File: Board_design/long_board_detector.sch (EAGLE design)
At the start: 57 parts, among them IC1 TL072P, IC2 78L05Z, IC3 LM393N, Q1 BC549, Q2 BC549, Q3 BC549, Q4 BC549, X1 22-23-2021, X2 22-23-2021

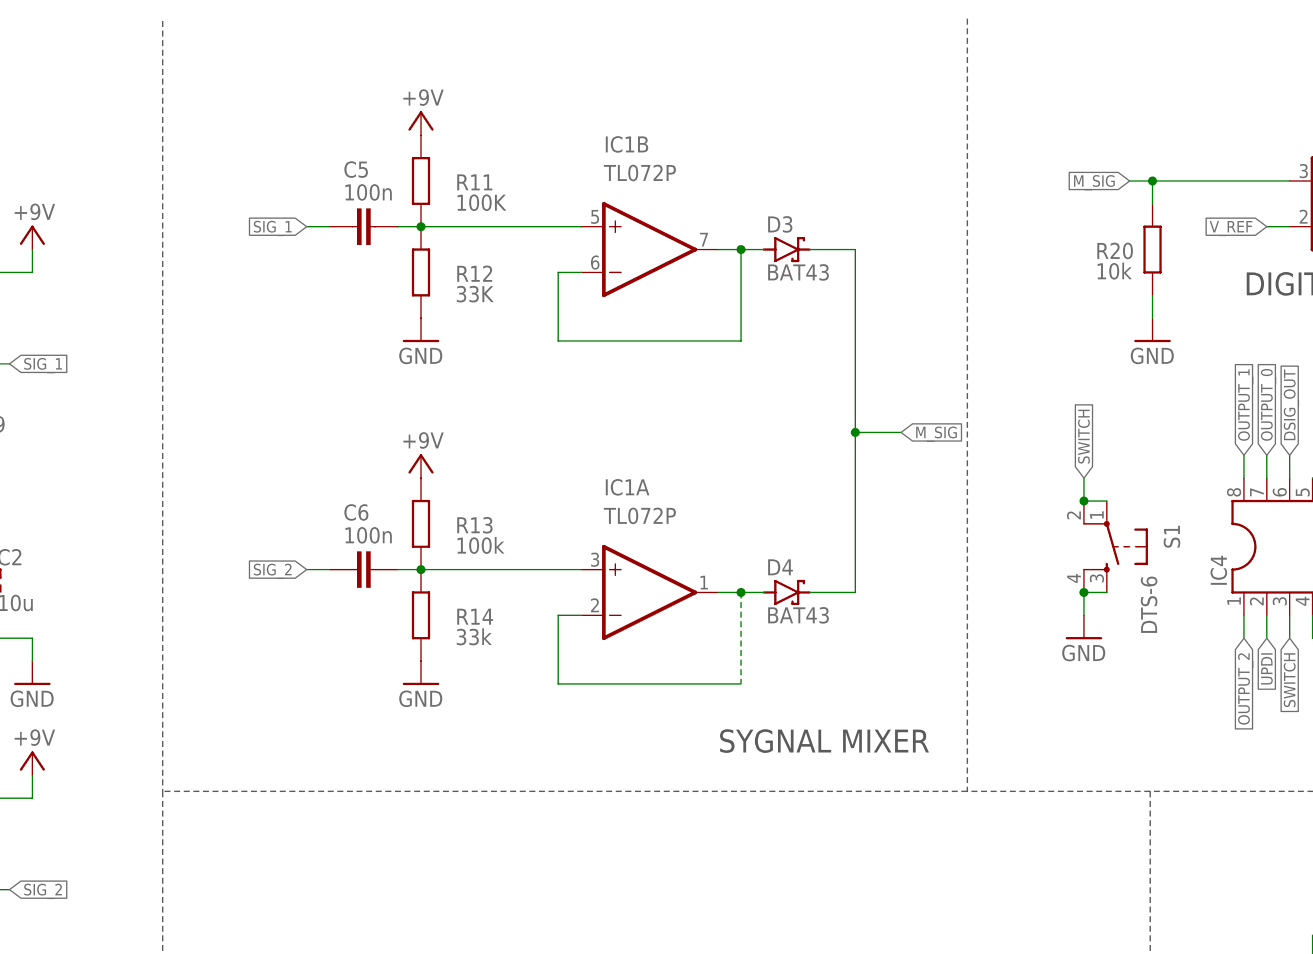
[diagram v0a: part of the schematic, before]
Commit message: Readme and brd design update
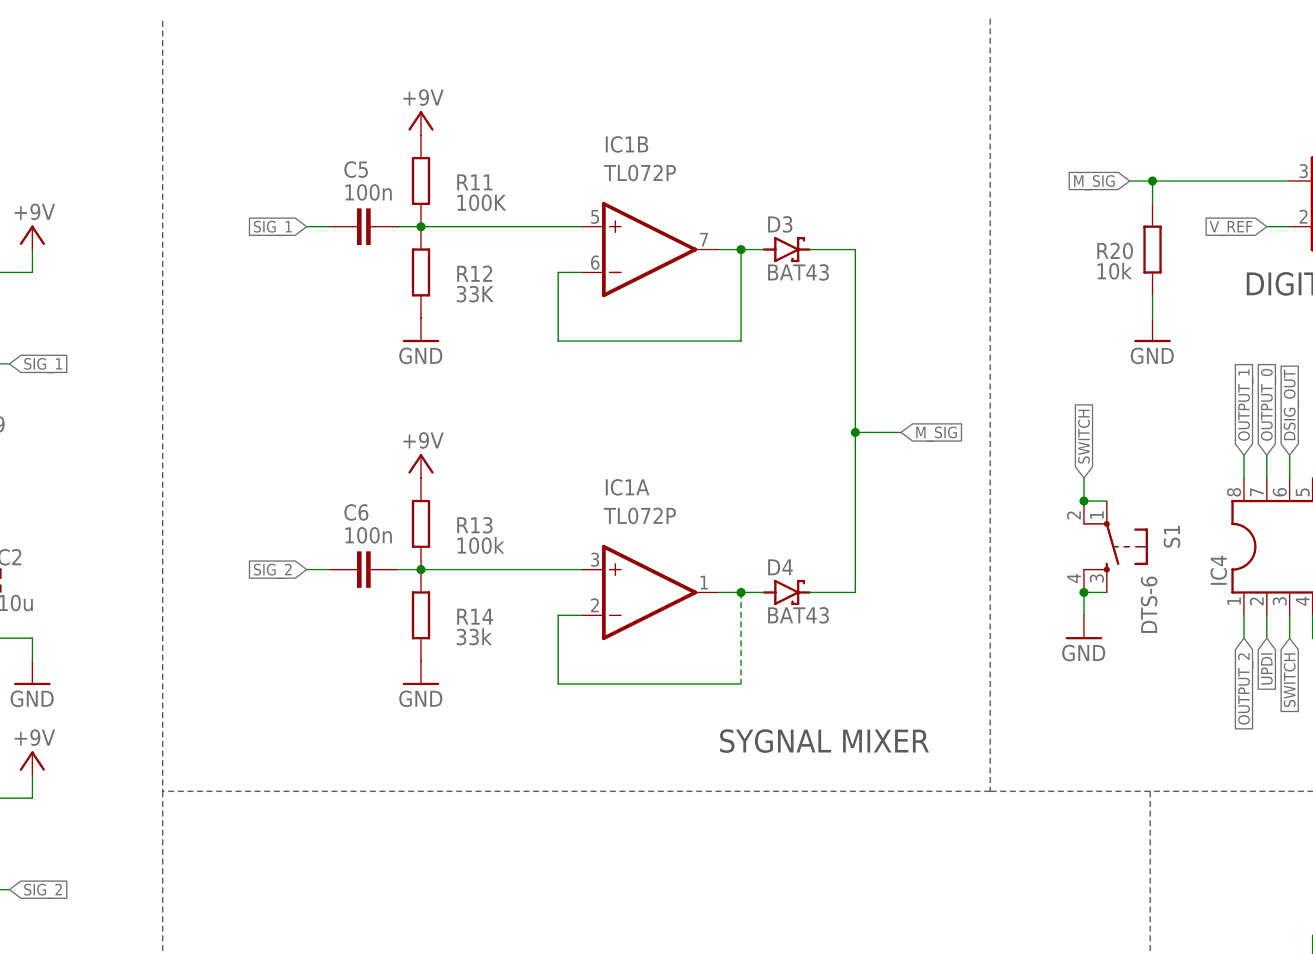
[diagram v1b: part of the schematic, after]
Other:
- note added: "this part of circut requires matel shielding (aluminum or copper)"
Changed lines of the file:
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@@
 <wire x1="70.358" y1="3.302" x2="70.358" y2="-82.55" width="0.1524" layer="97" style="longdash"/>
 <wire x1="238.76" y1="3.302" x2="180.086" y2="3.302" width="0.1524" layer="97" style="longdash"/>
-<wire x1="180.086" y1="3.302" x2="159.766" y2="3.302" width="0.1524" layer="97" style="longdash"/>
-<wire x1="159.766" y1="3.302" x2="70.358" y2="3.302" width="0.1524" layer="97" style="longdash"/>
-<wire x1="159.766" y1="89.154" x2="159.766" y2="3.302" width="0.1524" layer="97" style="longdash"/>
+<wire x1="180.086" y1="3.302" x2="162.306" y2="3.302" width="0.1524" layer="97" style="longdash"/>
+<wire x1="162.306" y1="3.302" x2="70.358" y2="3.302" width="0.1524" layer="97" style="longdash"/>
+<wire x1="162.306" y1="89.154" x2="162.306" y2="3.302" width="0.1524" layer="97" style="longdash"/>
 <wire x1="180.086" y1="3.302" x2="180.086" y2="-62.23" width="0.1524" layer="97" style="longdash"/>
 <text x="30.48" y="-78.74" size="2.54" layer="97">DETECTION HEAD x2</text>
@@
 Stanisław Lisek
 Marcin Kuśmierski</text>
+<wire x1="-10.16" y1="73.66" x2="-10.16" y2="-50.8" width="0.1524" layer="98"/>
+<wire x1="-10.16" y1="-50.8" x2="63.5" y2="-50.8" width="0.1524" layer="98"/>
+<wire x1="63.5" y1="-50.8" x2="63.5" y2="73.66" width="0.1524" layer="98"/>
+<wire x1="63.5" y1="73.66" x2="-10.16" y2="73.66" width="0.1524" layer="98"/>
+<text x="-7.62" y="-48.26" size="1.778" layer="98">this part of circut requires matel shielding (aluminum or copper)</text>
 </plain>
 <instances>
